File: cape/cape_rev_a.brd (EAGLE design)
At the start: 116.4 x 127.2 mm, 37 parts, among them U1 MAX3042BEUE, U10 MAX3042BEUE, U11 MAX3042BEUE, U12 MAX3042BEUE, U13 MAX3042BEUE, U14 MAX3042BEUE, U15 MAX3042BEUE, U16 MAX3042BEUE, U17 SN74LV245, U2 MAX3042BEUE, U3 MAX3042BEUE, U4 MAX3042BEUE, U5 MAX3042BEUE, U6 MAX3042BEUE, U7 MAX3042BEUE, U8 MAX3042BEUE, U9 MAX3042BEUE

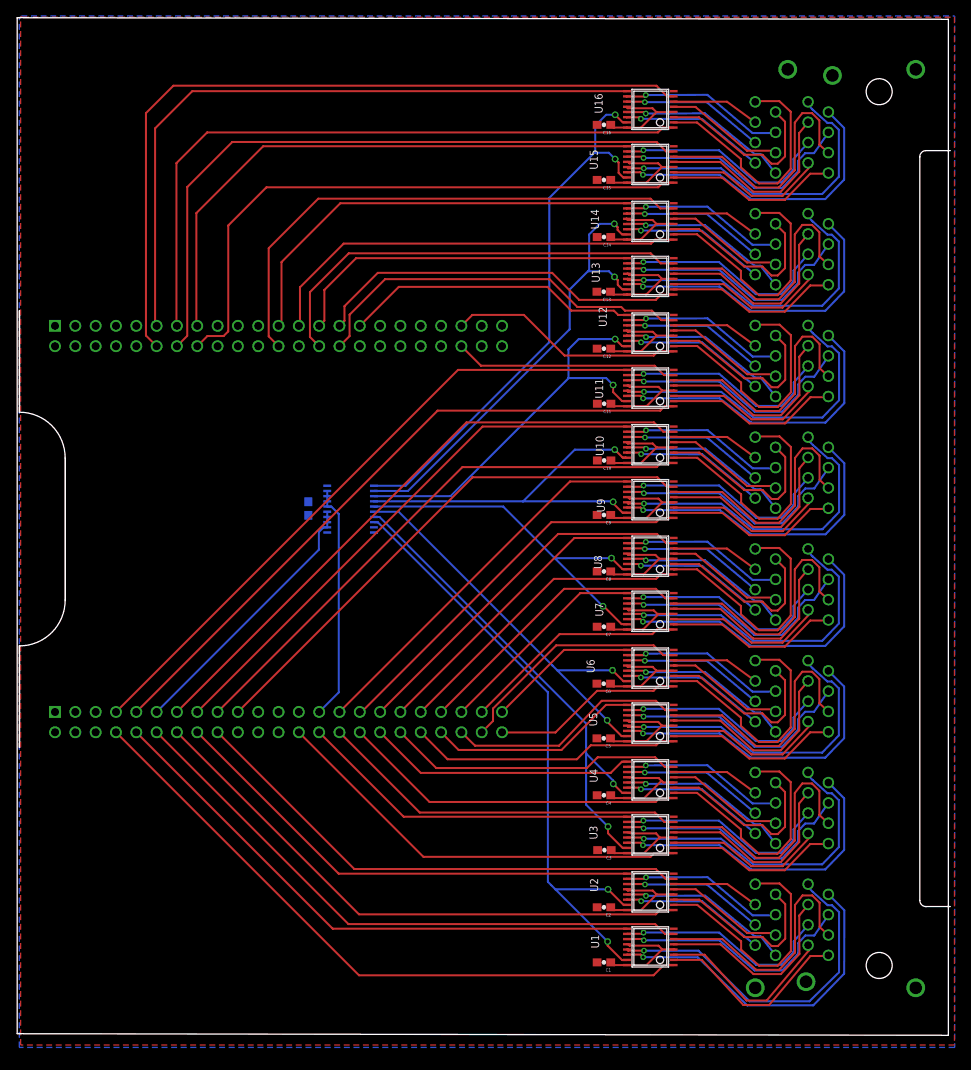
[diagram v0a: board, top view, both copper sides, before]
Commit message: Cape rev a
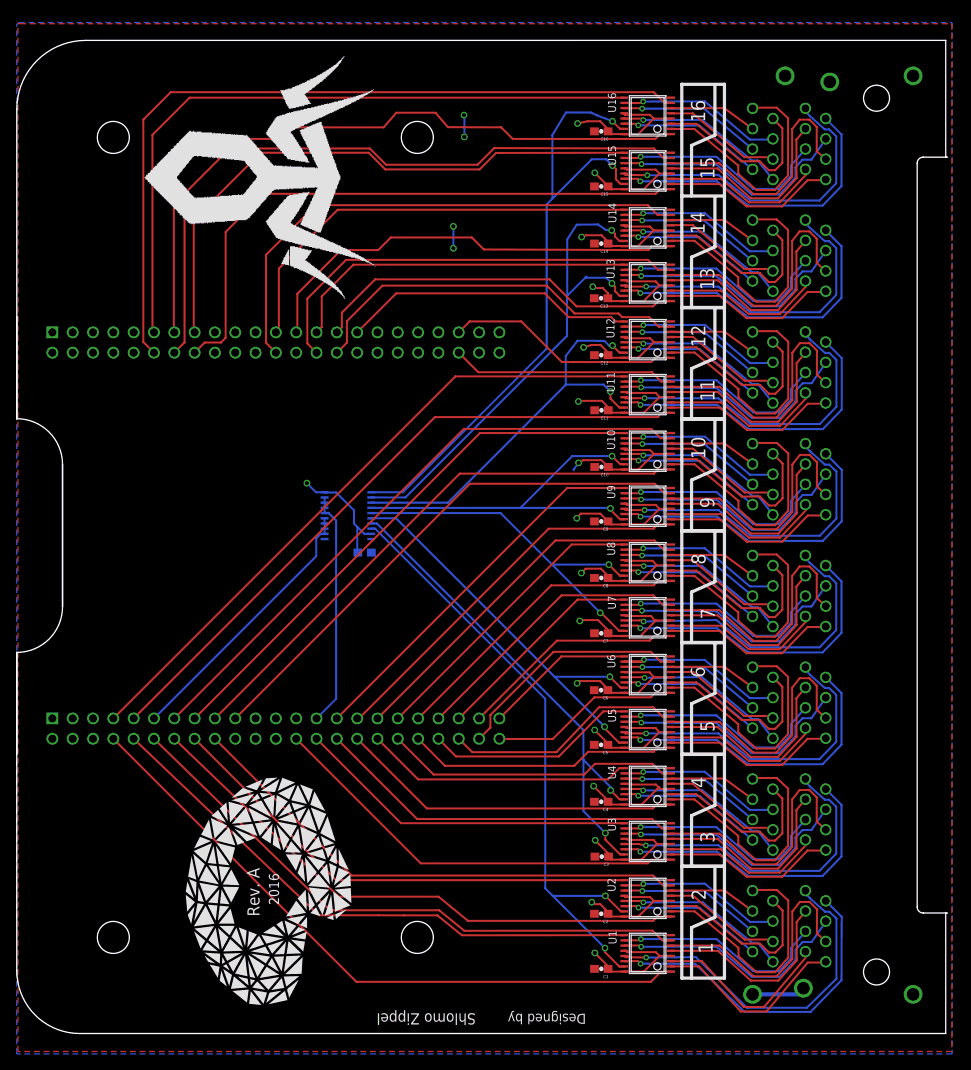
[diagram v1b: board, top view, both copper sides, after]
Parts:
- moved C17 8.94 mm to (43.4, 60.1), turned to 0 degrees
- moved U12 0.88 mm to (78.8, 86.7)
- moved C4 0.88 mm to (73.0, 29.0)
- moved C5 0.88 mm to (73.0, 36.1)
- moved C6 0.88 mm to (73.0, 42.9)
- moved C7 0.88 mm to (73.0, 50.0)
- moved C8 0.88 mm to (73.0, 56.9)
- moved C2 0.88 mm to (73.0, 15.0)
- moved U$2 0.88 mm to (101.1, 8.95)
- moved U$3 0.88 mm to (-14.7, 34.9)
- moved C1 0.88 mm to (73.0, 8.07)
- moved C3 0.88 mm to (73.1, 22.1)
- moved FRAME1 0.88 mm to (0.05, 24.0)
- moved U5 0.88 mm to (78.8, 38.0)
- moved U7 0.88 mm to (78.8, 52.0)
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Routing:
- net VCC: track 211.9 -> 270.9 mm, vias 0 -> 16
- net GND: track 0.00 -> 27.0 mm, vias 0 -> 5
- net CK1-4: track 69.8 -> 80.6 mm
- net CK1-3: track 57.9 -> 63.6 mm
- net S45: track 84.4 -> 87.2 mm
- net S44: track 71.4 -> 73.1 mm
- net S43: track 84.0 -> 85.8 mm
- net S39: track 54.1 -> 55.3 mm
- net CK1-2: track 51.3 -> 51.9 mm
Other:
- board size 116.4 x 127.2 mm -> 116.1 x 124.1 mm
- board text added: "1"
- board text added: "10"
- board text added: "11"
- board text added: "12"
- board text added: "13"
- board text added: "14"
- board text added: "15"
- board text added: "16"
- board text added: "2"
- board text added: "2016"
- board text added: "3"
- board text added: "4"
- board text added: "5"
- board text added: "6"
- board text added: "7"
- board text added: "8"
- board text added: "9"
- board text added: "Designed by"
- board text added: "Rev. A"
- board text added: "Shlomo Zippel"
